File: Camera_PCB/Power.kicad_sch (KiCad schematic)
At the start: 50 parts, among them J3 USB_C_Receptacle_PowerOnly_6P, Q3 AO3400A, Q4 AO3400A, SW2 SW_Push, U4 BQ297xy

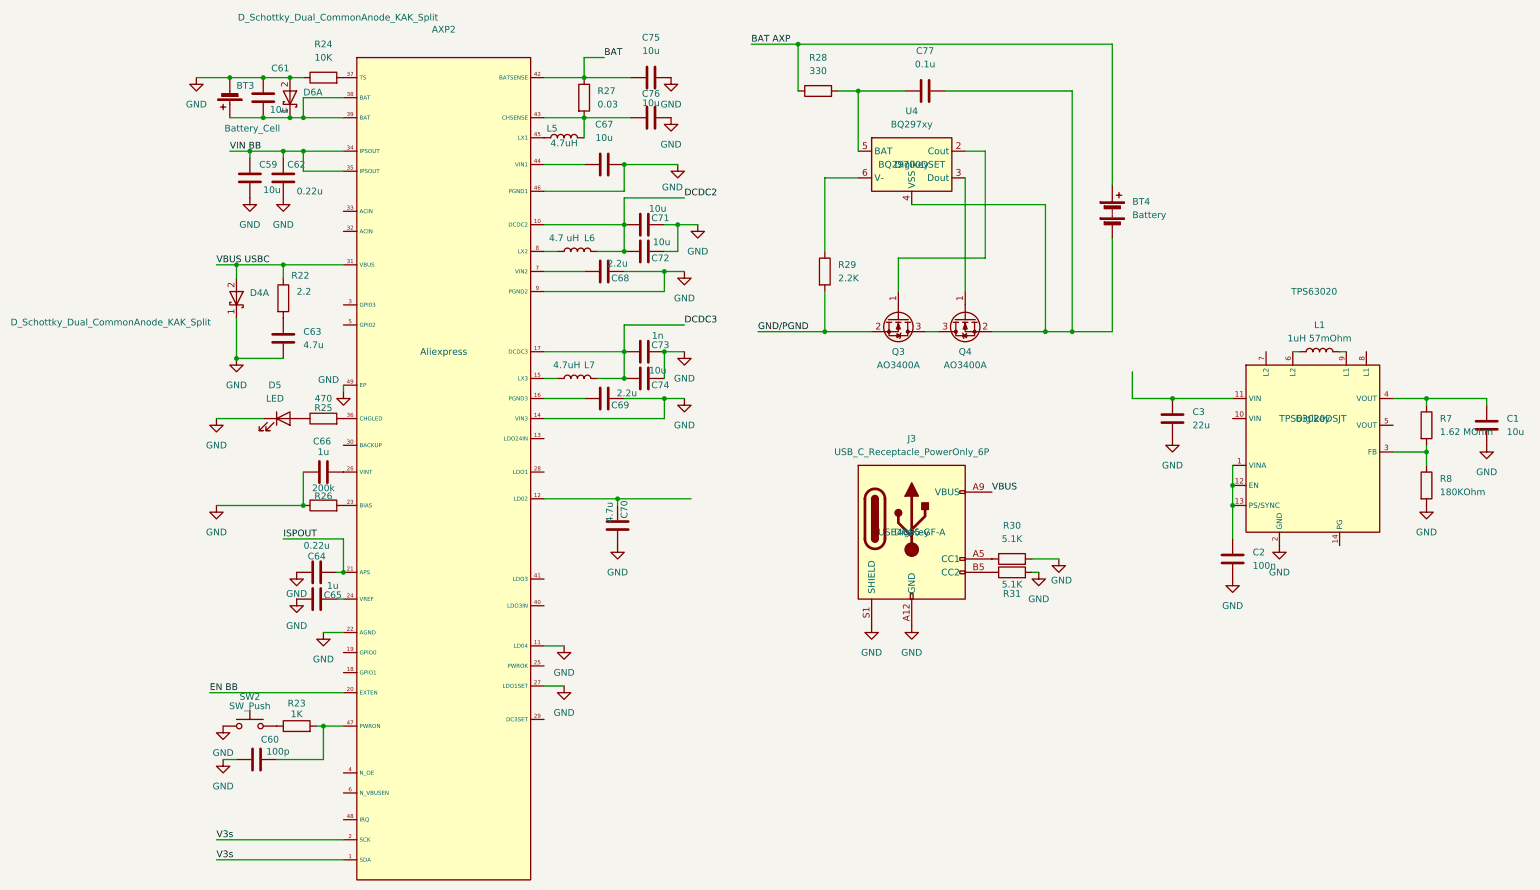
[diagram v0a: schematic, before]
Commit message: Camera PCB Schematic review 1
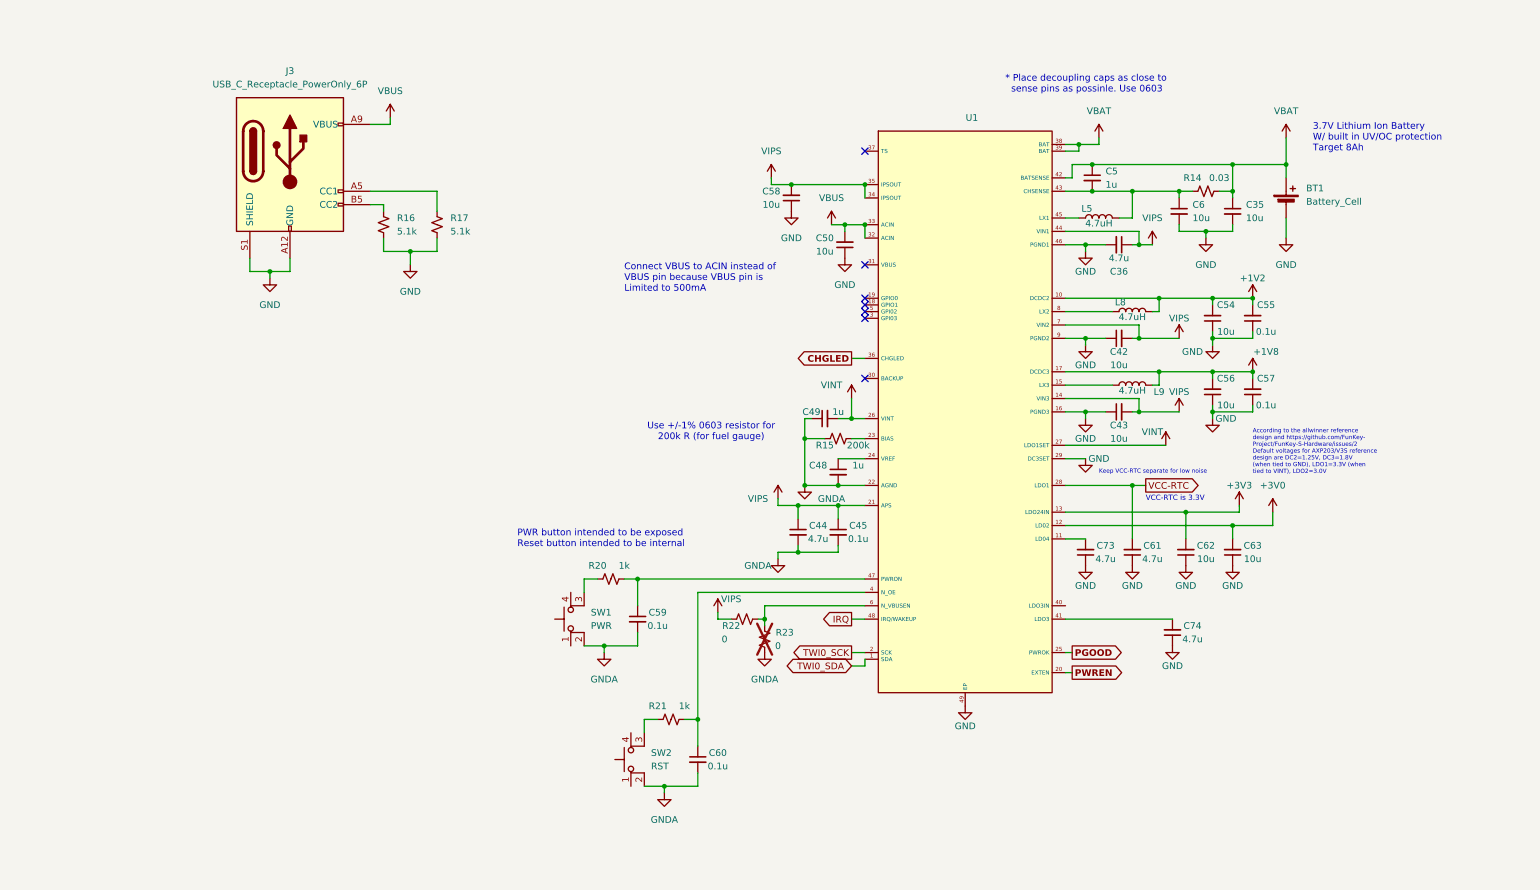
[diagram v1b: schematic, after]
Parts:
- removed BT3: Battery_Cell, symbol Device:Battery_Cell
- removed BT4: Battery, symbol Device:Battery
- removed C1, C59, C61, C67, C71, C72, C74, C75, C76: 10u, Capacitor_SMD:C_0805_2012Metric_Pad1.18x1.45mm_HandSolder, symbol Device:C
- removed C2: 100n, Capacitor_SMD:C_0603_1608Metric_Pad1.08x0.95mm_HandSolder, symbol Device:C
- removed C3: 22u, Capacitor_SMD:C_0805_2012Metric_Pad1.18x1.45mm_HandSolder, symbol Device:C
- removed C60: 100p, Capacitor_SMD:C_0603_1608Metric_Pad1.08x0.95mm_HandSolder, symbol Device:C
- removed C62, C64: 0.22u, Capacitor_SMD:C_0603_1608Metric_Pad1.08x0.95mm_HandSolder, symbol Device:C
- removed C63, C70: 4.7u, Capacitor_SMD:C_0805_2012Metric_Pad1.18x1.45mm_HandSolder, symbol Device:C
- removed C65, C66: 1u, Capacitor_SMD:C_0805_2012Metric_Pad1.18x1.45mm_HandSolder, symbol Device:C
- removed C68, C69: 2.2u, Capacitor_SMD:C_0805_2012Metric_Pad1.18x1.45mm_HandSolder, symbol Device:C
- removed C73: 1n, Capacitor_SMD:C_0603_1608Metric_Pad1.08x0.95mm_HandSolder, symbol Device:C
- removed C77: 0.1u, Capacitor_SMD:C_0603_1608Metric_Pad1.08x0.95mm_HandSolder, symbol Device:C
- removed D4, D6: D_Schottky_Dual_CommonAnode_KAK_Split, symbol Device:D_Schottky_Dual_CommonAnode_KAK_Split
- removed D5: LED, symbol Device:LED
- removed L1: 1uH 57mOhm, symbol Device:L
- removed L6: 4.7 uH, symbol Device:L
- removed L7: 4.7uH, symbol Device:L
- removed Q3, Q4: AO3400A, Package_TO_SOT_SMD:SOT-23, symbol Transistor_FET:AO3400A
- removed R22: 2.2, symbol Device:R
- removed R23: 1K, symbol Device:R
- removed R24: 10K, symbol Device:R
- removed R25: 470, symbol Device:R
- removed R26: 200k, symbol Device:R
- removed R27: 0.03, symbol Device:R
- removed R28: 330, symbol Device:R
- removed R29: 2.2K, symbol Device:R
- removed R30, R31: 5.1K, symbol Device:R
- removed R7: 1.62 MOhm, symbol Device:R
- removed R8: 180KOhm, symbol Device:R
- removed SW2: SW_Push, symbol Switch:SW_Push
- removed TPS63020: ~, BackupCamCustomParts:IC_TPS63020DSJT, symbol Senior:TPS63020
- removed U4: BQ297xy, Package_SON:WSON-6_1.5x1.5mm_P0.5mm, symbol Battery_Management:BQ297xy
- added BT1: Battery_Cell, symbol Device:Battery_Cell
- added C35, C42, C43, C50, C54, C56, C58, C6, C62, C63: 10u, symbol Device:C_Small
- added C36, C44, C61, C73, C74: 4.7u, symbol Device:C_Small
- added C45, C55, C57, C59, C60: 0.1u, symbol Device:C_Small
- added C48, C49, C5: 1u, symbol Device:C_Small
- added L8, L9: 4.7uH, symbol Device:L
- added R14: 0.03, symbol Device:R_Small_US
- added R15: 200k, symbol Device:R_Small_US
- added R16, R17: 5.1k, symbol Device:R_Small_US
- added R20, R21: 1k, symbol Device:R_Small_US
- added R22, R23: 0, symbol Device:R_Small_US
- added SW1: PWR, symbol Switch:SW_MEC_5E
- added SW2: RST, symbol Switch:SW_MEC_5E
- U1: renamed from AXP2; value ~ -> AXP203; symbol Senior:AXP203 -> custom_chips:AXP203; Distributor Aliexpress -> (none)
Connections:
- net BAT is gone; now on net VBAT: U1.42 (BATSENSE)
- net ISPOUT is gone; now on net VIPS: U1.21 (APS)
- net VIN BB is gone; now on net VIPS: U1.34 (IPSOUT), U1.35 (IPSOUT)
- net GND: now also U1.16 (PGND3), U1.29 (DC3SET), BT1.2 (-), C35.2, C36.2, C42.1, C43.1, C50.1, C54.1, C55.1, C56.1, C57.1, C58.1, C6.2, C61.1, C62.1, C63.1, C73.1, C74.1, R16.2, R17.2; no longer U1.11 (LD04), U1.14 (VIN3), U1.22 (AGND), U1.27 (LDO1SET)
- net VBUS: now also U1.32 (ACIN), U1.33 (ACIN), C50.2
- net at J3.A5 (CC1): now also R17.1
- net at J3.B5 (CC2): now also R16.1
- net VIPS: now reaches U1.7 (VIN2)
- net VIPS: now also U1.14 (VIN3), U1.44 (VIN1), C36.1, C42.2, C43.2, C44.1, C45.1, C58.2, R22.1
- net at U1.47 (PWRON): now also C59.1, R20.2
- net CHGLED: now reaches U1.36 (CHGLED)
- net at L5.2, U1.43 (CHSENSE): now also C5.2, C6.1, R14.1
- net VBAT: now reaches U1.38 (BAT), U1.39 (BAT)
- net VBAT: now also BT1.1 (+), C35.1, C5.1, R14.2
- net +3V0: now reaches U1.12 (LD02)
- net +3V0: now also C63.2
- net at U1.24 (VREF): now also C48.1
- net at U1.23 (BIAS): now also R15.2
- net +3V3: now reaches U1.13 (LDO24IN)
- net +3V3: now also C62.2
- net at U1.15 (LX3): now also L9.1
- net PGOOD: now reaches U1.25 (PWROK)
- net VINT: now reaches U1.26 (VINT)
- net VINT: now also U1.27 (LDO1SET), C49.2
- net VCC-RTC: now reaches U1.28 (LDO1)
- net VCC-RTC: now also C61.2
- net at U1.4 (N_OE): now also C60.1, R21.2
- net at U1.41 (LDO3): now also C74.2
- net IRQ: now reaches U1.48 (IRQ/WAKEUP)
- net at U1.6 (N_VBUSEN): now also R22.2, R23.2
- net at U1.8 (LX2): now also L8.1
- net DCDC2 renamed +1V2
- net +1V2: now also C54.2, C55.2, L8.2
- net DCDC3 renamed +1V8
- net +1V8: now also C56.2, C57.2, L9.2
- net EN BB renamed PWREN
- net V3s renamed TWI0_SCK
- net TWI0_SCK: no longer U1.1 (SDA)
- net VBUS USBC: no longer names the net of U1.31 (VBUS)
- new net: R21.1, SW2.3 (K)
- new net: C73.2, U1.11 (LD04)
- new net: R20.1, SW1.3 (K)
- new net GNDA: C44.2, C45.2, C48.2, C49.1, C59.2, C60.2, R15.1, R23.1, SW1.2, SW2.2, U1.22 (AGND)
- new net TWI0_SDA: U1.1 (SDA)
- no-connect marks 0 -> 7
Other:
- note added: "* Place decoupling caps as close to sense pins as possinle. Use 0603"
- note added: "3.7V Lithium Ion Battery W/ built in UV/OC protection Target 8Ah"
- note added: "According to the allwinner reference design and https://github.com/FunKey- Project/FunKey-S-Hardware/issues/2 Default voltages for AXP203/V3S reference design are DC2=1.25V, DC3=1.8V (when tied to GND), LDO1=3.3V (when tied to VINT), LDO2=3.0V"
- note added: "Connect VBUS to ACIN instead of VBUS pin because VBUS pin is Limited to 500mA"
- note added: "Keep VCC-RTC separate for low noise"
- note added: "PWR button intended to be exposed Reset button intended to be internal"
- note added: "Use +/-1% 0603 resistor for 200k R (for fuel gauge)"
- note added: "VCC-RTC is 3.3V"
- moved on the sheet: J3, L5, U1
